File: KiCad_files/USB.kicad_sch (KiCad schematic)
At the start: 3 parts, among them J2 USB4105-GF-A

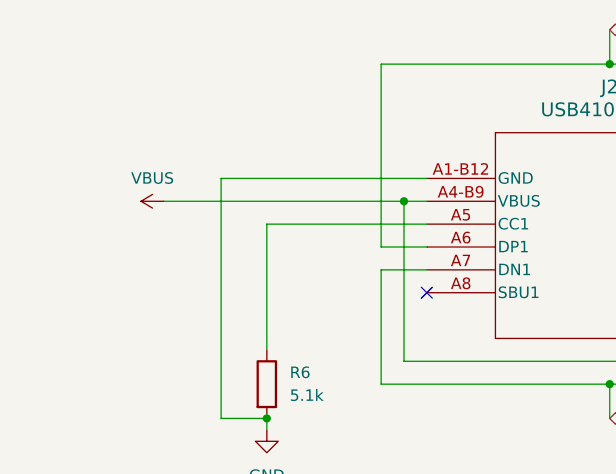
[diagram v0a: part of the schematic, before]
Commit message: johtoja
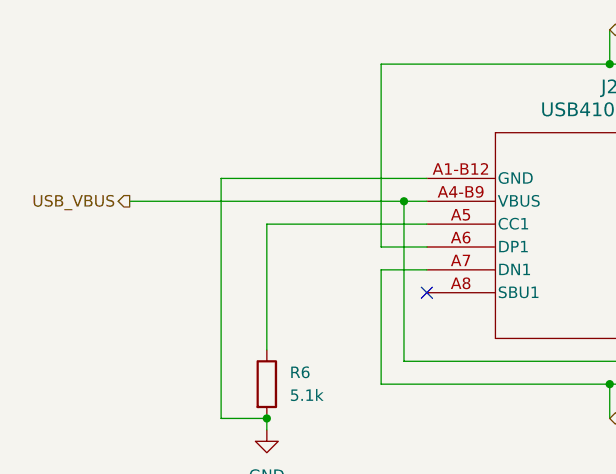
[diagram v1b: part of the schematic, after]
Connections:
- net VBUS renamed USB_VBUS
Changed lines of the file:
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@@
-	(wire
-		(pts
-			(xy 115.57 83.82) (xy 142.24 83.82)
-		)
-		(stroke
-			(width 0)
-			(type default)
-		)
-	)
 	(wire
 		(pts
@@
 	(wire
 		(pts
+			(xy 111.76 83.82) (xy 142.24 83.82)
+		)
+		(stroke
+			(width 0)
+			(type default)
+		)
+	)
+	(wire
+		(pts
 			(xy 127 109.22) (xy 127 107.95)
 		)
@@
 			(width 0)
 			(type default)
+		)
+	)
+	(hierarchical_label "USB_VBUS"
+		(shape output)
+		(at 111.76 83.82 180)
+		(effects
+			(font
+				(size 1.27 1.27)
+			)
+			(justify right)
 		)
 	)
@@
 					(unit 1)
 				)
-			)
-		)
-	)
-	(symbol
-		(lib_id "power:VBUS")
-		(at 115.57 83.82 90)
-		(unit 1)
-		(exclude_from_sim no)
-		(in_bom yes)
-		(on_board yes)
-		(dnp no)
-		(fields_autoplaced yes)
-		(property "Reference" "#PWR017"
-			(at 119.38 83.82 0)
-			(effects
-				(font
-					(size 1.27 1.27)
-				)
-				(hide yes)
-			)
-		)
-		(property "Value" "VBUS"
-			(at 114.3 81.28 90)
-			(effects
-				(font
-					(size 1.27 1.27)
-				)
-			)
-		)
-		(property "Footprint" ""
-			(at 115.57 83.82 0)
-			(effects
-				(font
-					(size 1.27 1.27)
-				)
-				(hide yes)
-			)
-		)
-		(property "Datasheet" ""
-			(at 115.57 83.82 0)
-			(effects
-				(font
-					(size 1.27 1.27)
-				)
-				(hide yes)
-			)
-		)
-		(property "Description" "Power symbol creates a global label with name \"VBUS\""
-			(at 115.57 83.82 0)
-			(effects
-				(font
-					(size 1.27 1.27)
-				)
-				(hide yes)
-			)
-		)
-		(pin "1"
-		)
-		(instances
-			(project "esp"
-				(path "/186d5500-054c-4b47-a89c-85f6ce2abe33/dce605b2-bfca-4721-a3b2-461c5c7ec909"
-					(reference "#PWR017")
-					(unit 1)
-				)
